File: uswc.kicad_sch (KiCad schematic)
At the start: 48 parts, among them J1 USB_C_Receptacle_USB2.0_16P, J2 Conn_01x02_Socket, P1 DFP, U1 ADG884xRM, U10 SRV05-4, U2 W25Q32JVZP, U3 SN74LVC1T45DBV, U4 RP2040, U5 XC6206PxxxMR, U6 74LVC1G125, U7 CH334F, U8 ADG884xRM, U9 SRV05-4, Y2 12MHz 10ppm

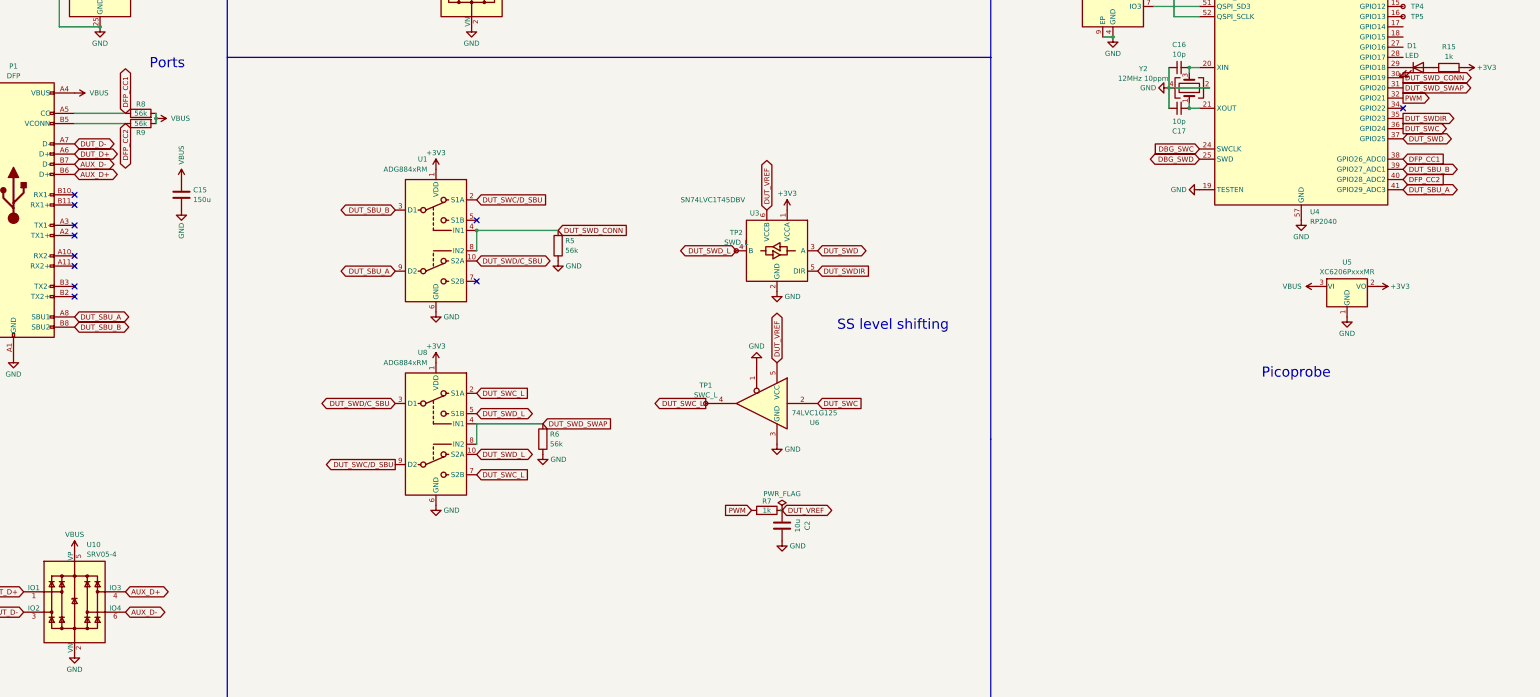
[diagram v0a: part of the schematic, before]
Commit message: v0.4
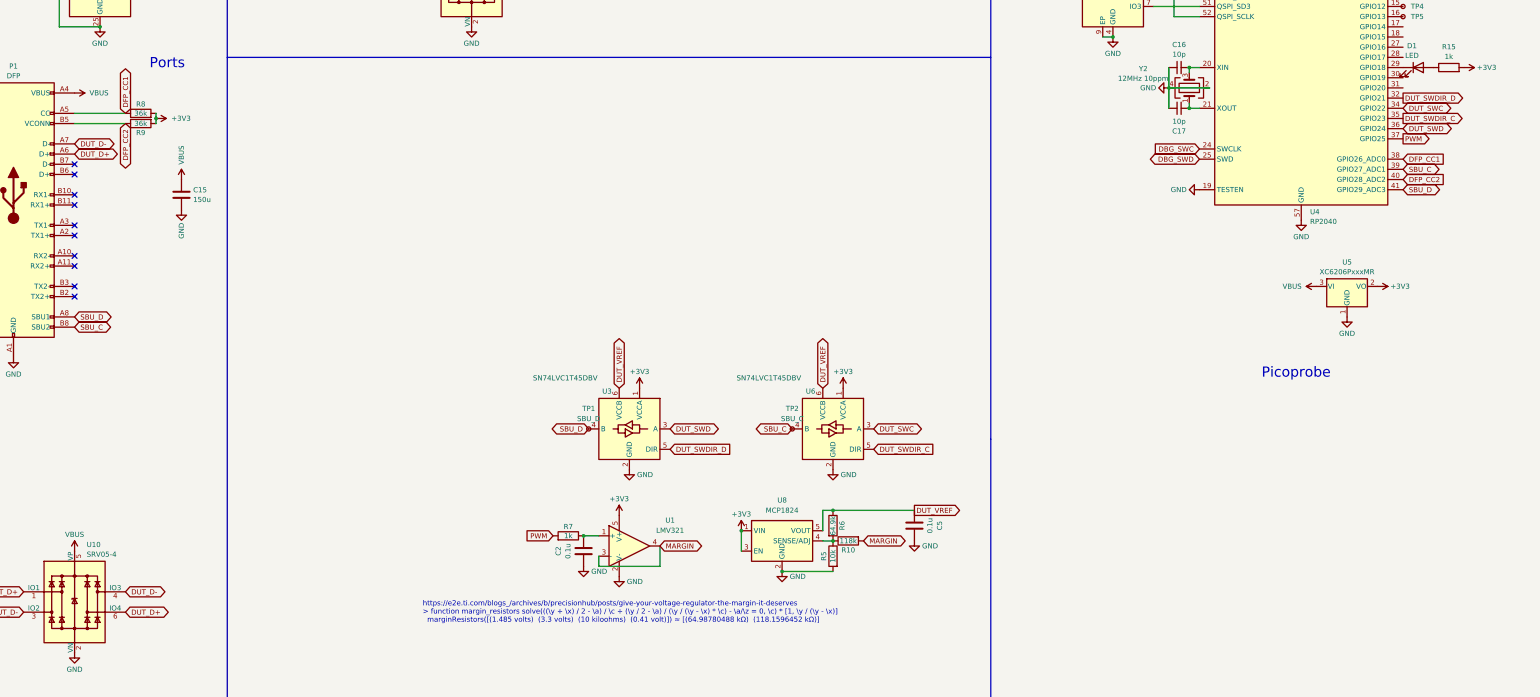
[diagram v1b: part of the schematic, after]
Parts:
- removed U1, U8: ADG884xRM, Package_SO:MSOP-10_3x3mm_P0.5mm, symbol Analog_Switch:ADG884xRM
- removed U6: 74LVC1G125, Package_TO_SOT_SMD:SOT-23-5, symbol 74xGxx:74LVC1G125
- added C5: 0.1u, Capacitor_SMD:C_0603_1608Metric, symbol Device:C
- added R10: 118k, Resistor_SMD:R_0603_1608Metric, symbol Device:R
- added U1: LMV321, Package_TO_SOT_SMD:SOT-353_SC-70-5, symbol Amplifier_Operational:LMV321
- added U6: SN74LVC1T45DBV, Package_TO_SOT_SMD:SOT-363_SC-70-6, symbol Logic_LevelTranslator:SN74LVC1T45DBV
- added U8: MCP1824, Package_TO_SOT_SMD:TSOT-23-5, symbol Regulator_Linear:ADP7142AUJZ
- C2: value 10u -> 0.1u
- R5: value 56k -> 10k
- R6: value 56k -> 64.9k
- R8, R9: value 56k -> 36k
- TP1: renamed from TP2; value SWD_L -> SBU_D
- TP2: renamed from TP1; value SWC_L -> SBU_C
- U2: footprint Package_SON:WSON-8-1EP_6x5mm_P1.27mm_EP3.4x4.3mm -> Package_SON:Winbond_USON-8-1EP_3x2mm_P0.5mm_EP0.2x1.6mm
- U3: footprint Package_TO_SOT_SMD:SOT-23-6 -> Package_TO_SOT_SMD:SOT-363_SC-70-6
- Y2: footprint Crystal:Crystal_SMD_3225-4Pin_3.2x2.5mm -> Crystal:Crystal_SMD_2016-4Pin_2.0x1.6mm
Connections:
- net DUT_SWC_L is gone; now on net SBU_C: TP2.1
- net DUT_SWD_L is gone; now on net SBU_D: TP1.1, U3.4 (B)
- net +3V3: now also R8.2, R9.2, U1.5 (V+), U6.1 (VCCA), U8.1 (VIN), U8.3 (EN)
- net DUT_D+: now also U10.6 (IO4)
- net DUT_D-: now also U10.4 (IO3)
- net DUT_SWC: now also U4.34 (GPIO22), U6.3 (A); no longer U4.36 (GPIO24)
- net DUT_SWD: now also U4.36 (GPIO24); no longer U4.37 (GPIO25)
- net DUT_VREF: now also R6.1, C5.1, U6.6 (VCCB), U8.5 (VOUT); no longer C2.1, R7.1
- net GND: now also R5.2, C5.2, U1.2 (V-), U6.2 (GND), U8.2 (GND); no longer R5.1, R6.1
- net PWM: now also U4.37 (GPIO25); no longer U4.32 (GPIO21)
- net VBUS: no longer R8.2, R9.2
- net AUX_D+: no longer names the net of P1.B6 (D+)
- net AUX_D+: no longer U10.4 (IO3)
- net AUX_D-: no longer names the net of P1.B7 (D-)
- net AUX_D-: no longer U10.6 (IO4)
- net DUT_SBU_A renamed SBU_D
- net DUT_SBU_B renamed SBU_C
- net SBU_C: now also U6.4 (B)
- net DUT_SWDIR renamed DUT_SWDIR_C
- net DUT_SWDIR_C: now also U6.5 (DIR); no longer U3.5 (DIR)
- net DUT_SWD_CONN: no longer names the net of U4.30 (GPIO19)
- net DUT_SWD_CONN: no longer R5.2
- net DUT_SWD_SWAP: no longer names the net of R6.2
- net DUT_SWD_SWAP: now also R5.1, R10.1, U8.4 (SENSE/ADJ); no longer U4.31 (GPIO20)
- new net: C2.1, R7.1, U1.1 (+)
- new net DUT_SWDIR_D: U3.5 (DIR), U4.32 (GPIO21)
- new net MARGIN: R10.2, U1.3 (-), U1.4
- no-connect marks 19 -> 18
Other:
- note added: "https://e2e.ti.com/blogs_/archives/b/precisionhub/posts/give-your-voltage-regulator-the-margin-it-deserves > function margin_resistors solve(((\y + \x) / 2 - \a) / \c + (\y / 2 - \a) / (\y / (\y - \x) * \c) - \a/\z = 0, \c) * [1, \y / (\y - \x)] marginResistors([(1.485 volts) (3.3 volts) (10 kiloohms) (0.41 volt)]) ≈ [(64.98780488 kΩ) (118.1596452 kΩ)]"
- note removed: "SS level shifting"
- moved on the sheet: C2, R7, TP1, TP2, U3
